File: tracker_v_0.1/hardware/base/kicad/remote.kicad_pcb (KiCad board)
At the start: 2 copper layers, 55.4 x 97.8 mm, 26 parts, among them J15 Conn_01x09_Female, J19 Conn_01x03_Female, J2 Conn_01x12_Female, J3 Conn_01x16_Female, J4 Conn_01x06_Female, J5 Conn_01x03_Female, J6 Conn_01x05_Female, Q1 Q_NMOS_GDS, Q3 Q_NPN_EBC, SW1 SW_Push, SW2 SW_Push, SW4 SW_Push_Dual, U1 RFM95HW

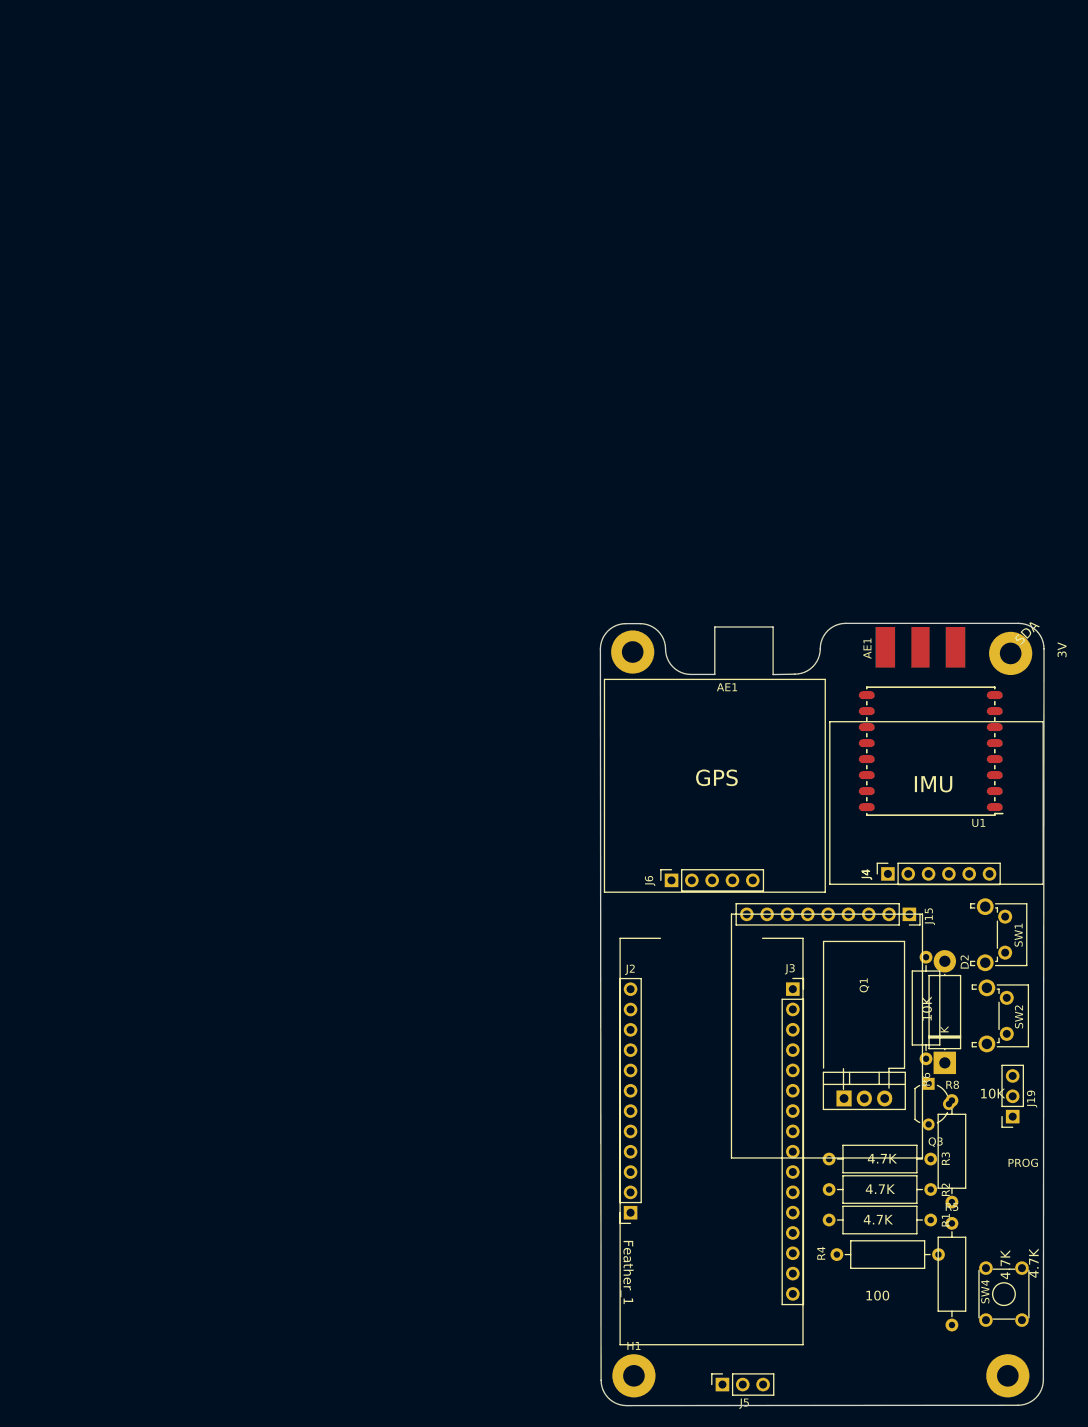
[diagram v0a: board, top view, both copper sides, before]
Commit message: reorg
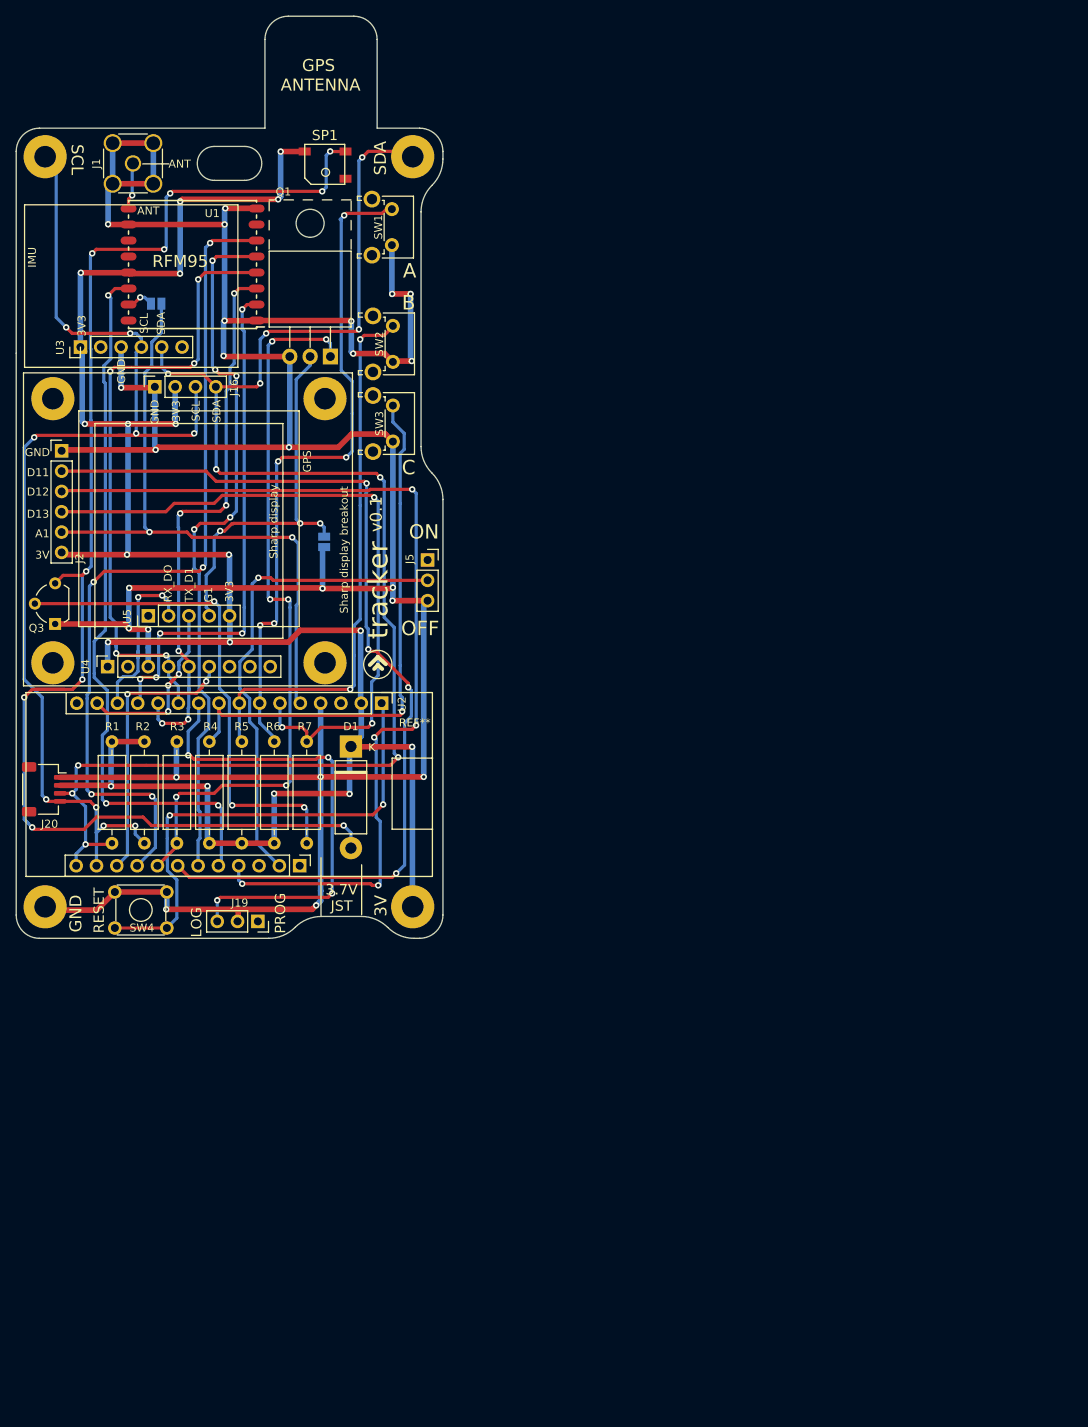
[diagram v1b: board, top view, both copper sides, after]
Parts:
- removed AE1: Antenna_Shield, digikey-footprints:RF_SMA_BoardEdge_142-0701-801
- removed D2: DIODE, Diode_THT:D_5W_P12.70mm_Horizontal
- removed J15: Conn_01x09_Female, Connector_PinSocket_2.54mm:PinSocket_1x09_P2.54mm_Vertical
- removed J3: Conn_01x16_Female, Connector_PinSocket_2.54mm:PinSocket_1x16_P2.54mm_Vertical
- removed J4: Conn_01x06_Female, Connector_PinSocket_2.54mm:PinSocket_1x06_P2.54mm_Vertical
- removed J6: Conn_01x05_Female, Connector_PinSocket_2.54mm:PinSocket_1x05_P2.54mm_Vertical
- removed R8: R, Resistor_THT:R_Axial_DIN0309_L9.0mm_D3.2mm_P12.70mm_Horizontal
- added D1: DIODE, Diode_THT:D_5W_P12.70mm_Horizontal, F.Cu at (10.1, 51.9)
- added J1: Conn_Coaxial, Connector_Coaxial:SMA_Amphenol_132134_Vertical, F.Cu at (-17.2, -21.0)
- added J16: Conn_01x04_Female, Connector_PinSocket_2.54mm:PinSocket_1x04_P2.54mm_Vertical, F.Cu at (-14.4, 6.93)
- added J20: Conn_01x04_Female, Connector_JST:JST_SH_SM04B-SRSS-TB_1x04-1MP_P1.00mm_Horizontal, F.Cu at (-28.3, 57.2)
- added JP1: Jumper_NO_Small, Jumper:SolderJumper-2_P1.3mm_Open_Pad1.0x1.5mm, B.Cu at (6.74, 26.3)
- added JP2: Jumper_NO_Small, Jumper:SolderJumper-2_P1.3mm_Open_Pad1.0x1.5mm, B.Cu at (-14.2, -3.46)
- added R7: R, Resistor_THT:R_Axial_DIN0309_L9.0mm_D3.2mm_P12.70mm_Horizontal, F.Cu at (4.57, 64.0)
- added SP1: SPEAKER_BUZZER5MM, Adafruit Circuit Playground:BUZZER_SMT_5MM, F.Cu at (6.82, -20.9)
- added SW3: SW_Push, Button_Switch_THT:SW_Tactile_SPST_Angled_PTS645Vx58-2LFS, F.Cu at (15.3, 9.27)
- added U2: feather, footprints:feather, F.Cu at (13.9, 46.5)
- added U3: Adafruit_IMU_BNO005, footprints:IMU_Ada_BNO005, F.Cu at (-23.7, 1.96)
- added U4: Adafruit_Sharp_Display_1_3, footprints:Display_adafruit_sharp_13, F.Cu at (0.00, 41.9)
- added U5: neo-6m-black, footprints:gps_neo6m_black, F.Cu at (-15.2, 35.6)
- J2: value Conn_01x12_Female -> Conn_01x06_Female; footprint Connector_PinSocket_2.54mm:PinSocket_1x12_P2.54mm_Vertical -> Connector_PinHeader_2.54mm:PinHeader_1x06_P2.54mm_Vertical
- Q1: footprint Package_TO_SOT_THT:TO-220-3_Vertical -> Package_TO_SOT_THT:TO-220-3_Horizontal_TabUp
- R3: value 4.7K -> 10K
- R5: value R -> 4.7K
- R6: value 10K -> 4.7K
- moved Q3 123.4 mm to (-26.9, 36.6), turned to 90 degrees
- moved J2 118.9 mm to (-26.1, 14.9), turned to 0 degrees
- moved R1 118.5 mm to (-19.8, 51.3), turned to 270 degrees
- moved SW1 117.0 mm to (15.2, -15.3)
- moved SW2 113.8 mm to (15.3, -0.69)
- moved SW4 113.5 mm to (-12.9, 74.6), turned to 180 degrees
- moved R2 113.1 mm to (-15.7, 51.3), turned to 270 degrees
- moved Q1 112.8 mm to (7.53, 3.15), turned to 180 degrees
- moved U1 110.5 mm to (-1.71, -1.35)
- moved J5 109.5 mm to (19.7, 28.6), turned to 0 degrees
- moved R3 102.2 mm to (-11.7, 64.0), turned to 90 degrees
- moved R5 100.7 mm to (-3.55, 64.0), turned to 90 degrees
- moved J19 97.5 mm to (-1.54, 73.8), turned to 270 degrees
- moved H5 97.0 mm to (17.8, -21.8)
- moved H6 96.1 mm to (-28.1, -21.8)
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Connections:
- net ~{RESET} renamed ~RESET
- H1 pad 1: unconnected-(H1-Pad1) -> GND
- J19 pad 1: unconnected-(J19-Pad1) -> (no net)
- J19 pad 2: Net-(J19-Pad2) -> GND
- J19 pad 3: A3 -> A5
- J2 pad 1: VBAT -> GND
- J2 pad 2: EN -> D10
- J2 pad 3: VBUS -> D13
- J2 pad 4: D13 -> A1
- J2 pad 5: D12 -> A0
- J2 pad 6: D11 -> +3V3
- J5 pad 1: GND -> (no net)
- J5 pad 2: VBAT -> EN
- J5 pad 3: VBAT_EXT -> GND
- R3 pad 1: +3V3 -> D9
- R3 pad 2: A5 -> GND
- R5 pad 1: Net-(J19-Pad2) -> +3V3
- R5 pad 2: GND -> A3
- R6 pad 1: D9 -> +3V3
- R6 pad 2: GND -> A2
- SW1 pad 1: A4 -> A2
- SW2 pad 1: A5 -> A3
- U1 pad 1: unconnected-(U1-Pad1) -> GND
- U1 pad 10: unconnected-(U1-Pad10) -> GND
- U1 pad 11: unconnected-(U1-Pad11) -> (no net)
- U1 pad 12: unconnected-(U1-Pad12) -> (no net)
- U1 pad 13: unconnected-(U1-Pad13) -> +3V3
- U1 pad 14: unconnected-(U1-Pad14) -> D12
- U1 pad 15: unconnected-(U1-Pad15) -> Net-(JP2-Pad1)
- U1 pad 16: unconnected-(U1-Pad16) -> (no net)
- U1 pad 2: unconnected-(U1-Pad2) -> MISO
- U1 pad 3: unconnected-(U1-Pad3) -> MOSI
- U1 pad 4: unconnected-(U1-Pad4) -> SCK
- U1 pad 5: unconnected-(U1-Pad5) -> D11
- U1 pad 6: unconnected-(U1-Pad6) -> D6
- U1 pad 7: unconnected-(U1-Pad7) -> (no net)
- U1 pad 8: unconnected-(U1-Pad8) -> GND
- U1 pad 9: unconnected-(U1-Pad9) -> Net-(J1-Pad1)
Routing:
- net GND: track 0.00 -> 408.4 mm, vias 0 -> 24
- net +3V3: track 0.00 -> 270.7 mm, vias 0 -> 18
- net SDA: track 0.00 -> 189.5 mm, vias 0 -> 11
- net Net-(D1-Pad2): track 0.00 -> 173.8 mm, vias 0 -> 10
- net SCL: track 0.00 -> 141.8 mm, vias 0 -> 9
- net D10: track 0.00 -> 119.4 mm, vias 0 -> 4
- net D13: track 0.00 -> 118.1 mm, vias 0 -> 5
- net D6: track 0.00 -> 105.8 mm, vias 0 -> 5
- net D9: track 0.00 -> 91.8 mm, vias 0 -> 6
- net D12: track 0.00 -> 90.7 mm, vias 0 -> 3
- net D11: track 0.00 -> 89.1 mm, vias 0 -> 5
- net A1: track 0.00 -> 85.6 mm, vias 0 -> 3
- net A2: track 0.00 -> 84.0 mm, vias 0 -> 5
- net A0: track 0.00 -> 80.1 mm, vias 0 -> 2
- net SCK: track 0.00 -> 78.0 mm, vias 0 -> 5
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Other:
- board size 55.4 x 97.8 mm -> 53.3 x 115.3 mm
- net class Default added: clearance 0.2, trace_width 0.25, via_dia 0.8, via_drill 0.4
- board text added: "3.7V"
- board text added: "3V3"
- board text added: "A"
- board text added: "A1"
- board text added: "ANT"
- board text added: "ANTENNA"
- board text added: "B"
- board text added: "C"
- board text added: "D11"
- board text added: "D12"
- board text added: "D13"
- board text added: "G1"
- board text added: "GND"
- board text added: "JST"
- board text added: "LOG"
- board text added: "OFF"
- board text added: "ON"
- board text added: "RESET"
- board text added: "RFM95"
- board text added: "RX_DO"
- board text added: "SCL"
- board text added: "Sharp display"
- board text added: "Sharp display breakout"
- board text added: "TX_D1"
- board text added: "pvos.org/tracker"
- board text added: "tracker"
- board text added: "tracker v0.1"
- board text added: "v0.1"
- board text removed: "100"
- board text removed: "10K"
- board text removed: "4.7K"
- board text removed: "Feather_1"
- board text removed: "Sharp Display"
